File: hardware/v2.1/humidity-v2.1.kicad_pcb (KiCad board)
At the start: 2 copper layers, 25 x 30 mm, 25 parts, among them P101 CON-SENSOR2, P102 DEBUG, P103 BOOT, U101 XMC1100-16, U102 HDC1080, U103 DRILL, U104 DRILL, U105 DRILL, U106 DRILL

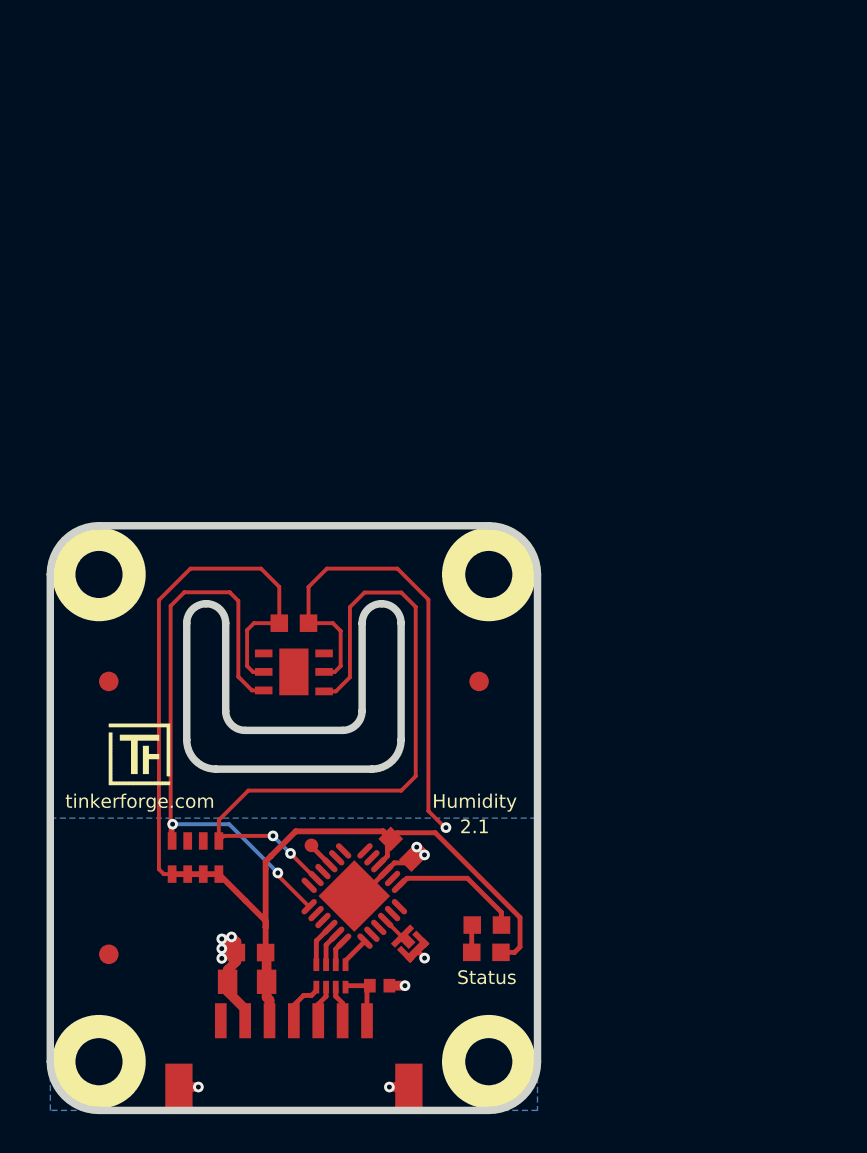
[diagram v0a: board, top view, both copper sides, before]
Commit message: new 25x25 design
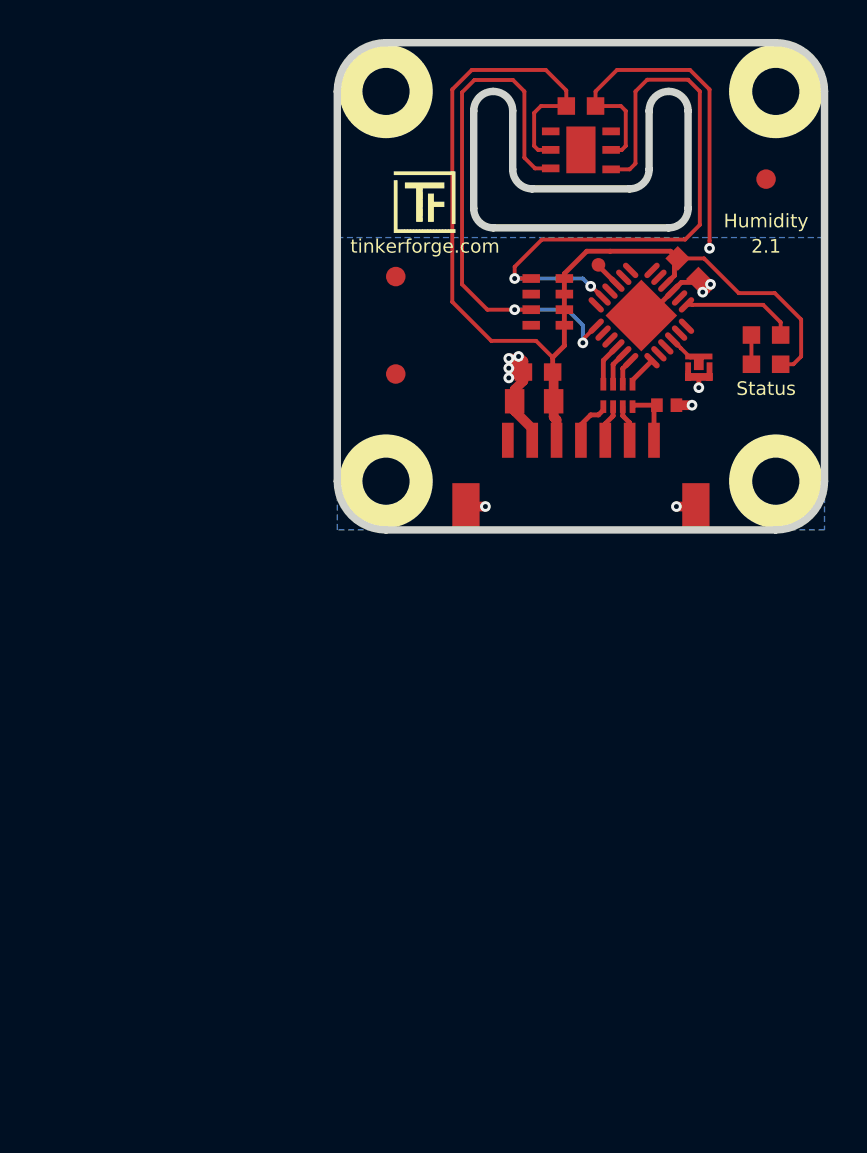
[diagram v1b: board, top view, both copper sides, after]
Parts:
- removed the Fiducial_Mark at (128.4, 150.3)
- removed the Fiducial_Mark at (147.4, 136.3)
- removed the Fiducial_Mark at (128.4, 136.3)
- added Fiducial_Mark: VAL**, kicad-libraries:Fiducial_Mark, F.Cu at (143.1, 120.5)
- added Fiducial_Mark: VAL**, kicad-libraries:Fiducial_Mark, F.Cu at (162.1, 110.5)
- added Fiducial_Mark: VAL**, kicad-libraries:Fiducial_Mark, F.Cu at (143.1, 115.5)
- moved RP102 33.8 mm to (150.9, 116.8), turned to 270 degrees
- moved R101 33.5 mm to (162.1, 118.5)
- moved D101 33.4 mm to (162.1, 120.0)
- moved C102 33.2 mm to (157.0, 122.1)
- moved C101 33.2 mm to (150.2, 121.9)
- moved C103 33.2 mm to (150.4, 120.4)
- moved C104 33.2 mm to (158.1, 115.1)
- moved P101 33.2 mm to (152.6, 128.5)
- moved P102 33.2 mm to (153.5, 114.9)
- moved RP101 33.2 mm to (154.5, 121.6)
- moved U101 33.2 mm to (155.7, 117.5)
- moved U103 33.2 mm to (162.6, 126.0)
- moved U104 33.2 mm to (142.6, 126.0)
- moved G*** 33.1 mm to (152.6, 119.8)
- moved VAL 33.1 mm to (146.6, 119.8)
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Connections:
- RP102 pad 7: Net-(RP102-Pad7) -> SCL
- RP102 pad 8: SCL -> Net-(RP102-Pad8)
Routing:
- net GND: track 46.7 -> 40.8 mm
- net VCC: track 62.6 -> 57.2 mm
- net SDA: track 36.0 -> 32.5 mm
- net SCL: track 31.2 -> 28.5 mm
- net Net-(R101-Pad1): track 6.76 -> 5.86 mm
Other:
- board size 25 x 30 mm -> 25 x 25 mm
- net class Default: clearance 0.149 -> 0.15
- rule trace_clearance: 0.149 -> 0.15
